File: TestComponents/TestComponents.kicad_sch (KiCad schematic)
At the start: 18 parts, among them J3V1 Conn_01x01_Male, J5 RFShield_OnePiece, J6 RFShield_OnePiece, U1 AD7991, U2 ADS1219

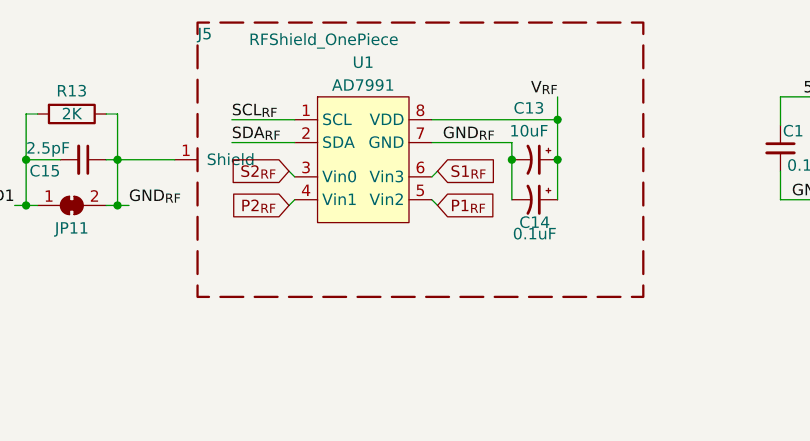
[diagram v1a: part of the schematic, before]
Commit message: SpectDrone Development
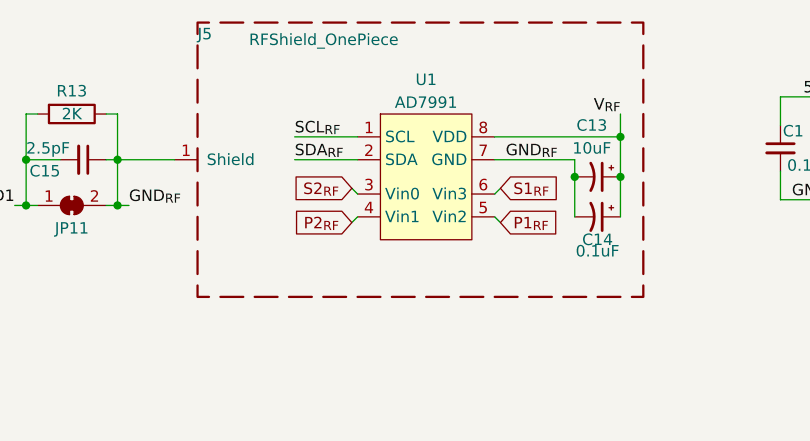
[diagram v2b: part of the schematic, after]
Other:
- moved on the sheet: C13, C14, U1

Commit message: SpectDrone Development
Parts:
- J3V1, JVIN1: Part Number (none) -> PH1-01-UA
- J5, J6: Part Number (none) -> BMI-S-101
- JP11, JP12: now left out of the parts list
- R13, R34: Part Number (none) -> ERJ-6ENF2001V
- R6: Part Number (none) -> ERA-6VRW1002V
- U1: Part Number (none) -> AD7991YRJZ-1500RL7
- U2: Part Number (none) -> ADS1219
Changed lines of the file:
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@@
+      (effects (font (size 1.27 1.27)) hide)
+    )
+    (property "Part Number" "BMI-S-101" (id 4) (at 51.435 35.56 0)
       (effects (font (size 1.27 1.27)) hide)
     )
@@
   )
   (symbol (lib_id "Jumper:SolderJumper_2_Bridged") (at 31.75 40.64 0) (mirror x) (unit 1)
-    (in_bom yes) (on_board yes)
+    (in_bom no) (on_board yes)
     (property "Reference" "JP12" (id 0) (at 31.75 43.18 0))
     (property "Value" "SolderJumper_2_Bridged" (id 1) (at 31.75 44.45 0)
@@
       (effects (font (size 1.27 1.27)) hide)
     )
+    (property "Part Number" "PH1-01-UA" (id 4) (at 126.365 106.045 0)
+      (effects (font (size 1.27 1.27)) hide)
+    )
     (pin "1")
   )
@@
   )
   (symbol (lib_id "Jumper:SolderJumper_2_Bridged") (at 110.49 40.64 0) (mirror x) (unit 1)
-    (in_bom yes) (on_board yes)
+    (in_bom no) (on_board yes)
     (property "Reference" "JP11" (id 0) (at 110.49 43.18 0))
     (property "Value" "SolderJumper_2_Bridged" (id 1) (at 110.49 44.45 0)
@@
       (effects (font (size 1.27 1.27)) hide)
     )
+    (property "Part Number" "ERJ-6ENF2001V" (id 4) (at 31.75 30.48 0)
+      (effects (font (size 1.27 1.27)) hide)
+    )
     (pin "1")
     (pin "2")
@@
     )
     (property "Datasheet" "https://www.analog.com/media/en/technical-documentation/data-sheets/AD7991_7995_7999.pdf" (id 3) (at 149.86 26.67 0)
+      (effects (font (size 1.27 1.27)) hide)
+    )
+    (property "Part Number" "AD7991YRJZ-1500RL7" (id 4) (at 149.86 26.67 0)
       (effects (font (size 1.27 1.27)) hide)
     )
@@
     )
     (property "Datasheet" "http://www.ti.com/lit/ds/symlink/ads1219.pdf" (id 3) (at 72.39 57.15 0)
+      (effects (font (size 1.27 1.27)) hide)
+    )
+    (property "Part Number" "ADS1219" (id 4) (at 72.39 46.99 0)
       (effects (font (size 1.27 1.27)) hide)
     )
@@
       (effects (font (size 1.27 1.27)) hide)
     )
+    (property "Part Number" "ERA-6VRW1002V" (id 4) (at 80.01 30.48 0)
+      (effects (font (size 1.27 1.27)) hide)
+    )
     (pin "1")
     (pin "2")
@@
     )
     (property "Datasheet" "~" (id 3) (at 134.62 35.56 0)
+      (effects (font (size 1.27 1.27)) hide)
+    )
+    (property "Part Number" "BMI-S-101" (id 4) (at 132.08 35.56 0)
       (effects (font (size 1.27 1.27)) hide)
     )
@@
       (effects (font (size 1.27 1.27)) hide)
     )
+    (property "Part Number" "PH1-01-UA" (id 4) (at 126.365 114.3 0)
+      (effects (font (size 1.27 1.27)) hide)
+    )
     (pin "1")
   )
@@
       (effects (font (size 1.27 1.27)) hide)
     )
+    (property "Part Number" "ERJ-6ENF2001V" (id 4) (at 110.49 30.48 0)
+      (effects (font (size 1.27 1.27)) hide)
+    )
